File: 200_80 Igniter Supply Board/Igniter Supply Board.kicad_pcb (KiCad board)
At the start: 2 copper layers, 80 x 49 mm, 3 parts

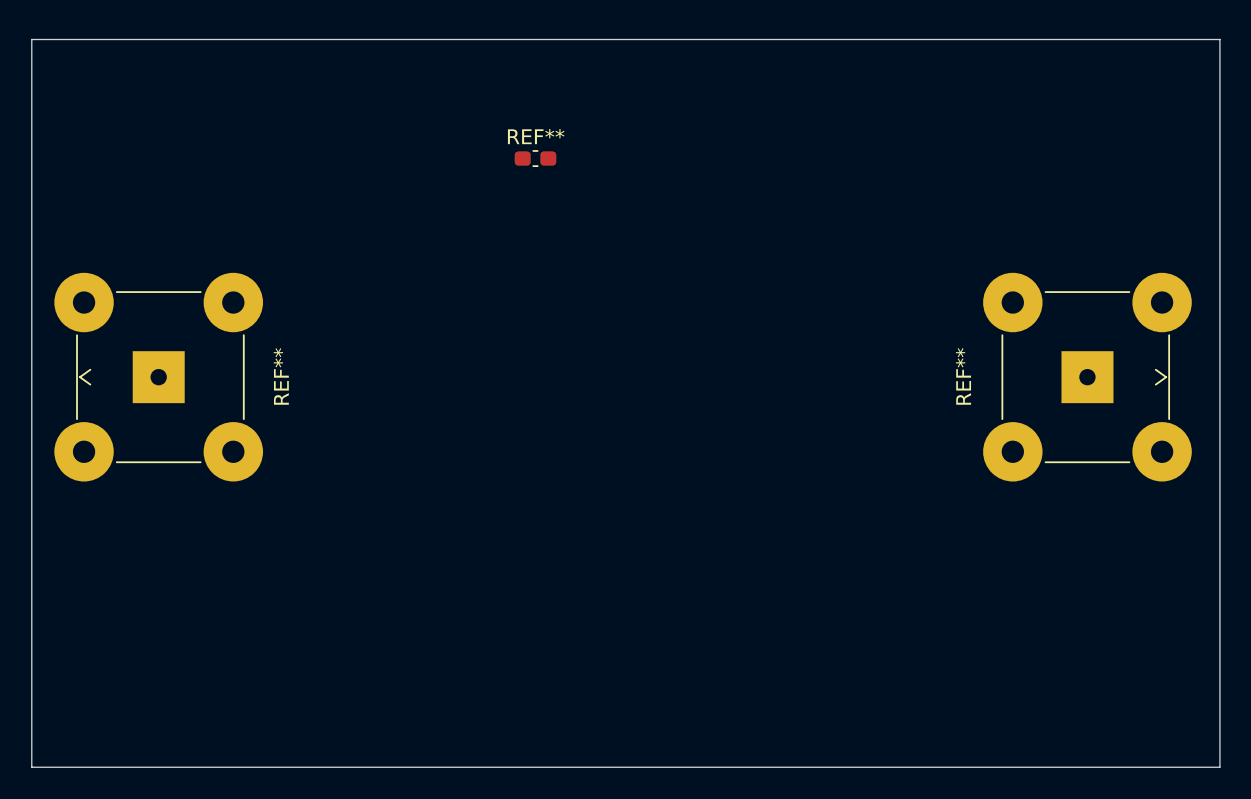
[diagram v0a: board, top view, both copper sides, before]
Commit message: Igniter PCB floorplan
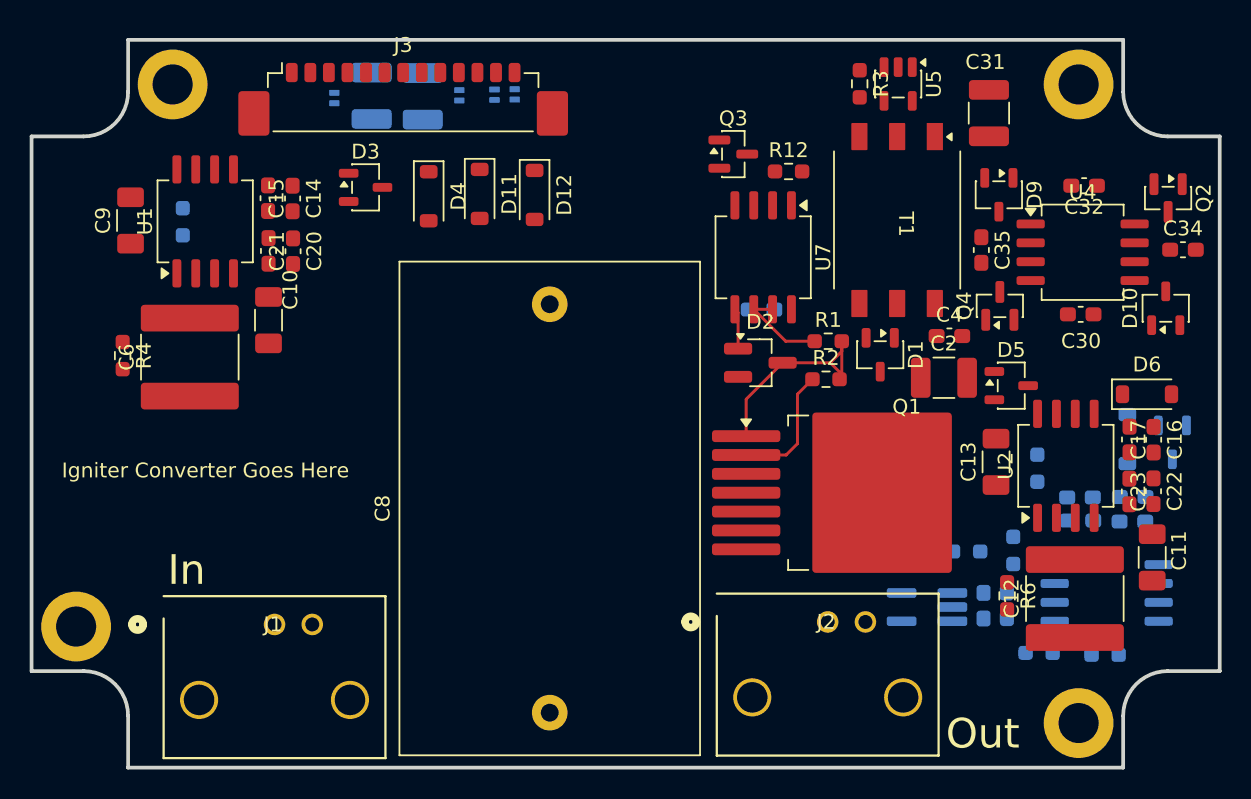
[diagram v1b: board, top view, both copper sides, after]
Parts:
- removed REF** (x2): BNC_TEConnectivity_1478035_Horizontal, Connector_Coaxial:BNC_TEConnectivity_1478035_Horizontal
- removed REF**: C_0603_1608Metric_Pad1.08x0.95mm_HandSolder, Capacitor_SMD:C_0603_1608Metric_Pad1.08x0.95mm_HandSolder
- added ?: , , F.Cu at (163.6, 129.2)
- added ?: , , F.Cu at (163.6, 86.2)
- added ?: , , F.Cu at (102.6, 86.2)
- added C10: 470pF, Capacitor_SMD:C_1206_3216Metric_Pad1.33x1.80mm_HandSolder, F.Cu at (109.0, 102.1)
- added C11: 470pF, Capacitor_SMD:C_1206_3216Metric_Pad1.33x1.80mm_HandSolder, F.Cu at (168.5, 118.0)
- added C12: 1pF, Capacitor_SMD:C_2225_5664Metric_Pad1.80x6.60mm_HandSolder, F.Cu at (163.3, 120.8)
- added C13: 470pF, Capacitor_SMD:C_1206_3216Metric_Pad1.33x1.80mm_HandSolder, F.Cu at (158.0, 111.6)
- added C14: 100nF, Capacitor_SMD:C_0603_1608Metric_Pad1.08x0.95mm_HandSolder, F.Cu at (110.6, 93.9)
- added C15: 1nF, Capacitor_SMD:C_0603_1608Metric_Pad1.08x0.95mm_HandSolder, F.Cu at (109.0, 93.9)
- added C16: 100nF, Capacitor_SMD:C_0603_1608Metric_Pad1.08x0.95mm_HandSolder, F.Cu at (168.6, 110.1)
- added C17: 1nF, Capacitor_SMD:C_0603_1608Metric_Pad1.08x0.95mm_HandSolder, F.Cu at (167.0, 110.1)
- added C18: 100nF, Capacitor_SMD:C_0603_1608Metric_Pad1.08x0.95mm_HandSolder, B.Cu at (163.7, 114.0)
- added C19: 1nF, Capacitor_SMD:C_0603_1608Metric_Pad1.08x0.95mm_HandSolder, B.Cu at (163.7, 115.6)
- added C2: 10uF, Capacitor_SMD:C_1210_3225Metric_Pad1.33x2.70mm_HandSolder, F.Cu at (154.5, 106.0)
- added C20: 100nF, Capacitor_SMD:C_0603_1608Metric_Pad1.08x0.95mm_HandSolder, F.Cu at (110.7, 97.4)
- added C21: 1nF, Capacitor_SMD:C_0603_1608Metric_Pad1.08x0.95mm_HandSolder, F.Cu at (109.0, 97.4)
- added C22: 100nF, Capacitor_SMD:C_0603_1608Metric_Pad1.08x0.95mm_HandSolder, F.Cu at (168.6, 113.6)
- added C23: 1nF, Capacitor_SMD:C_0603_1608Metric_Pad1.08x0.95mm_HandSolder, F.Cu at (167.0, 113.6)
- added C24: 100nF, Capacitor_SMD:C_0603_1608Metric_Pad1.08x0.95mm_HandSolder, B.Cu at (167.2, 115.6)
- added C25: 1nF, Capacitor_SMD:C_0603_1608Metric_Pad1.08x0.95mm_HandSolder, B.Cu at (167.2, 114.0)
- added C26: 100nF, Capacitor_SMD:C_0603_1608Metric_Pad1.08x0.95mm_HandSolder, B.Cu at (158.7, 121.3)
- added C27: 1nF, Capacitor_SMD:C_0603_1608Metric_Pad1.08x0.95mm_HandSolder, B.Cu at (157.2, 121.3)
- added C28: 10uF, Capacitor_SMD:C_1210_3225Metric_Pad1.33x2.70mm_HandSolder, B.Cu at (116.0, 87.0)
- added C29: 10uF, Capacitor_SMD:C_1210_3225Metric_Pad1.33x2.70mm_HandSolder, B.Cu at (119.4, 87.0)
- added C30: 100nF, Capacitor_SMD:C_0603_1608Metric_Pad1.08x0.95mm_HandSolder, F.Cu at (163.7, 101.7)
- added C31: 10uF, Capacitor_SMD:C_1210_3225Metric_Pad1.33x2.70mm_HandSolder, F.Cu at (157.5, 88.1)
- added C32: 1nF, Capacitor_SMD:C_0603_1608Metric_Pad1.08x0.95mm_HandSolder, F.Cu at (163.9, 93.0)
- added C34: 1nF, Capacitor_SMD:C_0603_1608Metric_Pad1.08x0.95mm_HandSolder, F.Cu at (170.6, 97.3)
- added C35: 1nF, Capacitor_SMD:C_0603_1608Metric_Pad1.08x0.95mm_HandSolder, F.Cu at (157.0, 97.3)
- added C4: 100nF, Capacitor_SMD:C_0603_1608Metric_Pad1.08x0.95mm_HandSolder, F.Cu at (154.9, 103.1)
- added C5: 1nF, Capacitor_SMD:C_0603_1608Metric_Pad1.08x0.95mm_HandSolder, B.Cu at (142.2, 101.4)
- added C6: 1pF, Capacitor_SMD:C_2225_5664Metric_Pad1.80x6.60mm_HandSolder, F.Cu at (103.7, 104.6)
- added C8: 1uF, Capacitor_THT:C_Rect_L33.0mm_W20.0mm_P27.50mm_MKS4, F.Cu at (128.0, 128.5)
- added C9: 470pF, Capacitor_SMD:C_1206_3216Metric_Pad1.33x1.80mm_HandSolder, F.Cu at (99.7, 95.4)
- added D1: BAT54L, Package_TO_SOT_SMD:SOT-23-3, F.Cu at (150.2, 104.4)
- added D10: BAT54L, Package_TO_SOT_SMD:SOT-23-3, F.Cu at (169.4, 101.3)
- added D11: MMSZ4685, Diode_SMD:D_SOD-123, F.Cu at (123.2, 93.6)
- added D12: MMSZ4685, Diode_SMD:D_SOD-123, F.Cu at (126.9, 93.6)
- added D13: PESD3V3U1UL, Diode_SMD:D_SOD-882, B.Cu at (124.2, 86.9)
- added D14: PESD5V0S1UL, Diode_SMD:D_SOD-882, B.Cu at (113.4, 87.1)
- added D15: PESD5V0S1UL, Diode_SMD:D_SOD-882, B.Cu at (121.9, 86.9)
- added D16: PESD3V3U1UL, Diode_SMD:D_SOD-882, B.Cu at (125.6, 86.9)
- added D2: SZBZX84C18LT3G, Package_TO_SOT_SMD:SOT-23_Handsoldering, F.Cu at (142.1, 104.9)
- added D3: BAT54L, Package_TO_SOT_SMD:SOT-23-3, F.Cu at (115.5, 93.1)
- added D4: MMSZ4685, Diode_SMD:D_SOD-123, F.Cu at (119.8, 93.7)
- added D5: BAT54L, Package_TO_SOT_SMD:SOT-23-3, F.Cu at (159.0, 106.5)
- added D6: MMSZ4685, Diode_SMD:D_SOD-123, F.Cu at (168.2, 107.1)
- added D7: BAT54L, Package_TO_SOT_SMD:SOT-23-3, B.Cu at (169.9, 110.3)
- added D8: MMSZ4685, Diode_SMD:D_SOD-123, B.Cu at (166.8, 110.1)
- added D9: BAT54L, Package_TO_SOT_SMD:SOT-23-3, F.Cu at (158.2, 93.6)
- added H3: M2.5, MountingHole:MountingHole_2.7mm_M2.5_DIN965_Pad, F.Cu at (96.1, 122.7)
- added J1: BNC, 0_PAY_Footprint_Library:CONN_73138-5033_MOL, F.Cu at (109.4, 122.6)
- added J2: BNC, 0_PAY_Footprint_Library:CONN_73138-5033_MOL, F.Cu at (146.7, 122.4)
- added J3: 53261-1371, Connector_Molex:Molex_PicoBlade_53398-1371_1x13-1MP_P1.25mm_Vertical, F.Cu at (118.1, 86.7)
- added Q1: G2R1000MT33J-TR, Package_TO_SOT_SMD:TO-263-7_TabPin8, F.Cu at (148.8, 113.7)
- added Q2: BSS123, Package_TO_SOT_SMD:SOT-23, F.Cu at (169.6, 93.8)
- added Q3: BSS123, Package_TO_SOT_SMD:SOT-23, F.Cu at (140.3, 90.9)
- added Q4: BSS123, Package_TO_SOT_SMD:SOT-23, F.Cu at (158.3, 101.1)
- added R1: 0R, Resistor_SMD:R_0603_1608Metric_Pad0.98x0.95mm_HandSolder, F.Cu at (146.7, 103.5)
- added R10: 1k, Resistor_SMD:R_0603_1608Metric_Pad0.98x0.95mm_HandSolder, B.Cu at (160.9, 124.5)
- added R11: 2.7k, Resistor_SMD:R_0603_1608Metric_Pad0.98x0.95mm_HandSolder, B.Cu at (159.2, 117.6)
- added R12: 370R, Resistor_SMD:R_0603_1608Metric_Pad0.98x0.95mm_HandSolder, F.Cu at (144.0, 92.1)
- added R2: DNP, Resistor_SMD:R_0603_1608Metric_Pad0.98x0.95mm_HandSolder, F.Cu at (146.6, 106.0)
- added R3: 165k, Resistor_SMD:R_0603_1608Metric_Pad0.98x0.95mm_HandSolder, F.Cu at (148.8, 86.2)
- added R4: 4.53M, Resistor_SMD:R_0603_1608Metric_Pad0.98x0.95mm_HandSolder, F.Cu at (99.2, 104.5)
- added R5: 10k, Resistor_SMD:R_0603_1608Metric_Pad0.98x0.95mm_HandSolder, B.Cu at (103.2, 95.4)
- added R6: 4.53M, Resistor_SMD:R_0603_1608Metric_Pad0.98x0.95mm_HandSolder, F.Cu at (158.7, 120.6)
- added R7: 10k, Resistor_SMD:R_0603_1608Metric_Pad0.98x0.95mm_HandSolder, B.Cu at (160.8, 112.0)
- added R8: 1k, Resistor_SMD:R_0603_1608Metric_Pad0.98x0.95mm_HandSolder, B.Cu at (156.0, 117.6)
- added R9: 2.5k, Resistor_SMD:R_0603_1608Metric_Pad0.98x0.95mm_HandSolder, B.Cu at (165.3, 124.6)
- added T1: 750319697, 0_PAY_Footprint_Library:Transformer_Wuerth_750319697, F.Cu at (151.4, 95.6)
- added TH1: NCU18XH103F60RB, Resistor_SMD:R_0603_1608Metric_Pad0.98x0.95mm_HandSolder, B.Cu at (150.2, 114.0)
- added U1: OP37, Package_SO:SOIC-8_5.3x6.2mm_P1.27mm, F.Cu at (104.8, 95.4)
- added U2: OP37, Package_SO:SOIC-8_5.3x6.2mm_P1.27mm, F.Cu at (162.7, 111.9)
- added U3: OP37, Package_SO:SOIC-8_5.3x6.2mm_P1.27mm, B.Cu at (165.4, 120.4)
- added U4: LMP2012, Package_SO:SOIC-8_5.3x6.2mm_P1.27mm, F.Cu at (163.8, 97.5)
- added U5: LT8301, Package_TO_SOT_SMD:TSOT-23-5, F.Cu at (151.4, 86.2)
- added U6: ~, Package_TO_SOT_SMD:TSOT-23-5_HandSoldering, B.Cu at (153.3, 121.4)
- added U7: Si8261BAC, Package_SO:SOIC-8_5.3x6.2mm_P1.27mm, F.Cu at (142.3, 97.8)
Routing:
- net Net-(D2-K): track 0.00 -> 14.6 mm
- net Net-(D2-A): track 0.00 -> 11.3 mm
- net Net-(R1-Pad1): track 0.00 -> 6.26 mm
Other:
- outline, holes or cut-outs redrawn
- board text added: "Arthur Prudius"
- board text added: "Igniter Breakout"
- board text added: "Igniter Converter Goes Here"
- board text added: "In"
- board text added: "Out"
- board text added: "Rev 1.0"
